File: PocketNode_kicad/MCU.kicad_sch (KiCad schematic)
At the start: 8 parts, among them U3 ESP32-S3-WROOM-1-N16R8

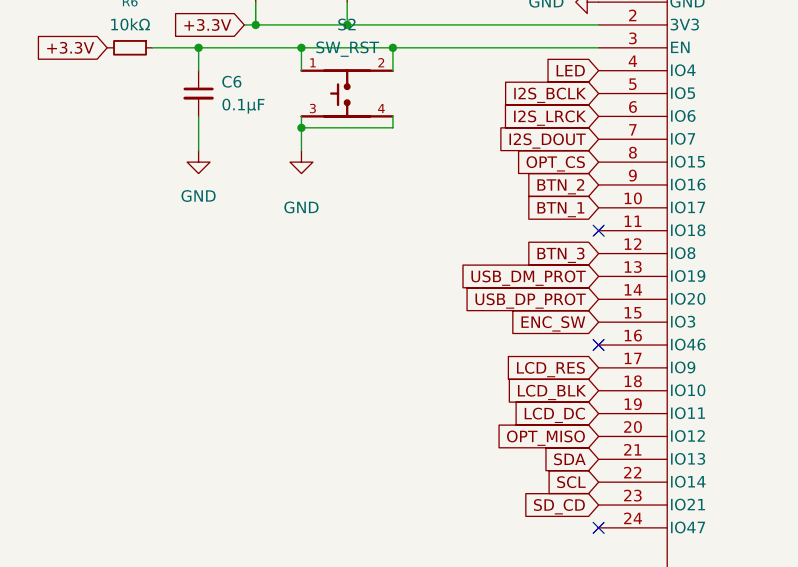
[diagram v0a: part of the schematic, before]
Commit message: update11
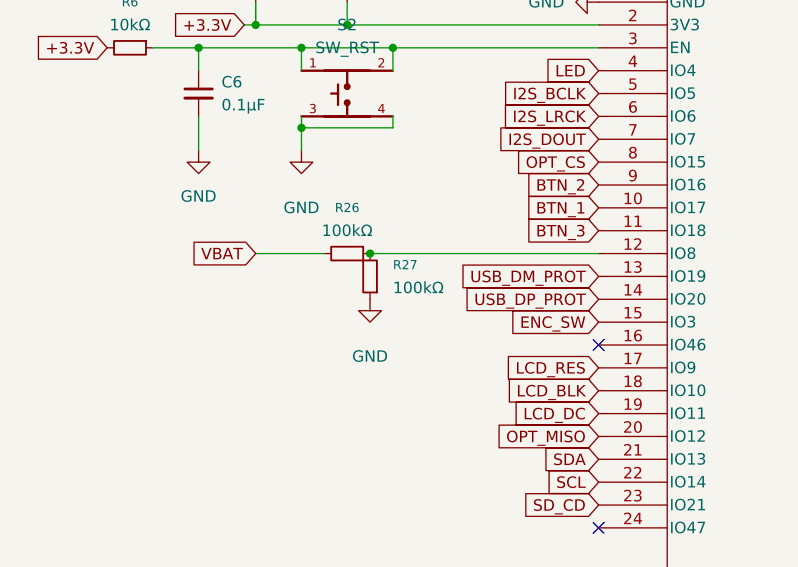
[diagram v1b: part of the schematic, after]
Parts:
- added R26, R27: 100kΩ, Resistor_SMD:R_0603_1608Metric_Pad0.98x0.95mm_HandSolder, symbol Device:R_Small
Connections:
- net BTN_3: now also U3.11 (IO18); no longer U3.12 (IO8)
- net GND: now also R27.1
- new net: R26.1, R27.2, U3.12 (IO8)
- new net VBAT: R26.2
- no-connect marks 9 -> 8
